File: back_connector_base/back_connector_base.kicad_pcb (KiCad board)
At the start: 2 copper layers, 102 x 77.7 mm, 10 parts, among them J1 Conn_01x12_Pin, J10 Conn_01x04_Socket, J2 Conn_01x16_Pin, J3 Conn_01x03_Socket, J4 Conn_01x03_Socket, J5 Conn_01x03_Socket, J6 Conn_01x03_Socket, J7 Conn_01x04_Socket, J8 Conn_01x04_Socket, J9 Conn_01x04_Socket

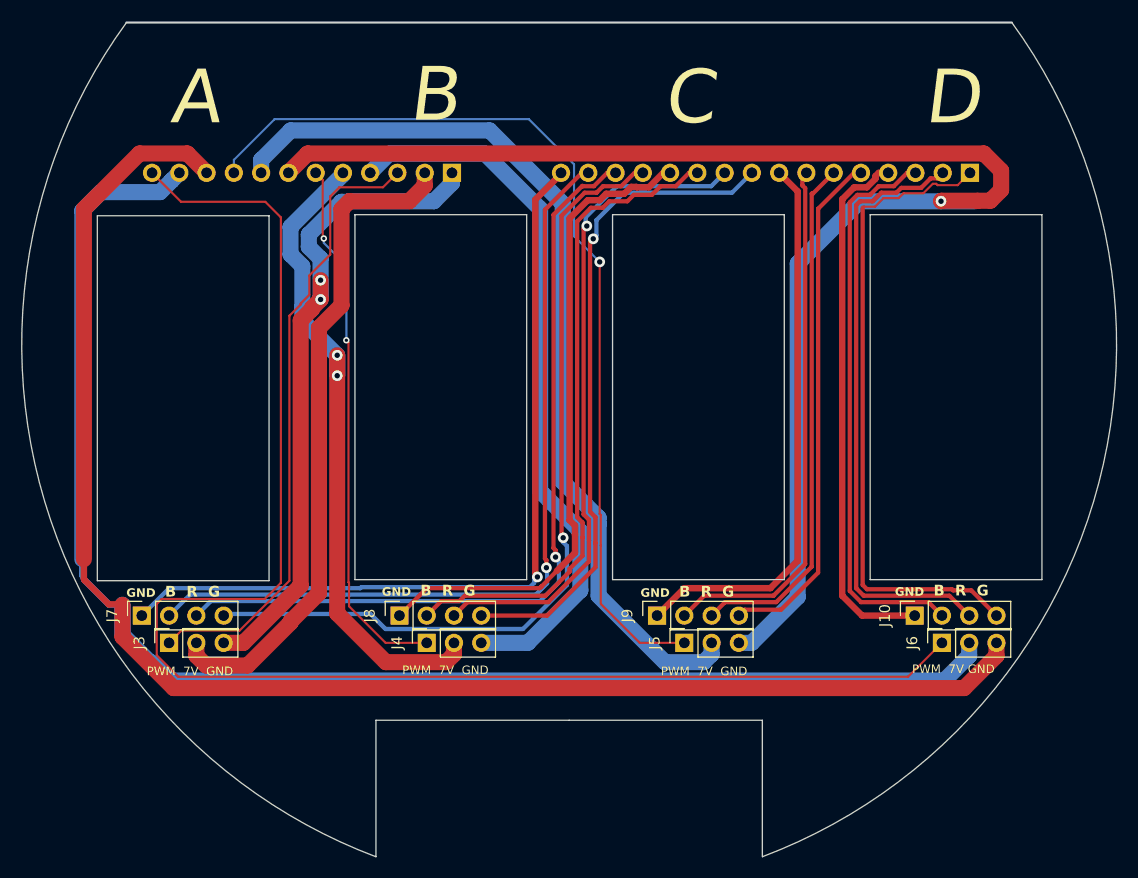
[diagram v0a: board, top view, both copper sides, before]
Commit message: ESC周りの配線用基板進捗
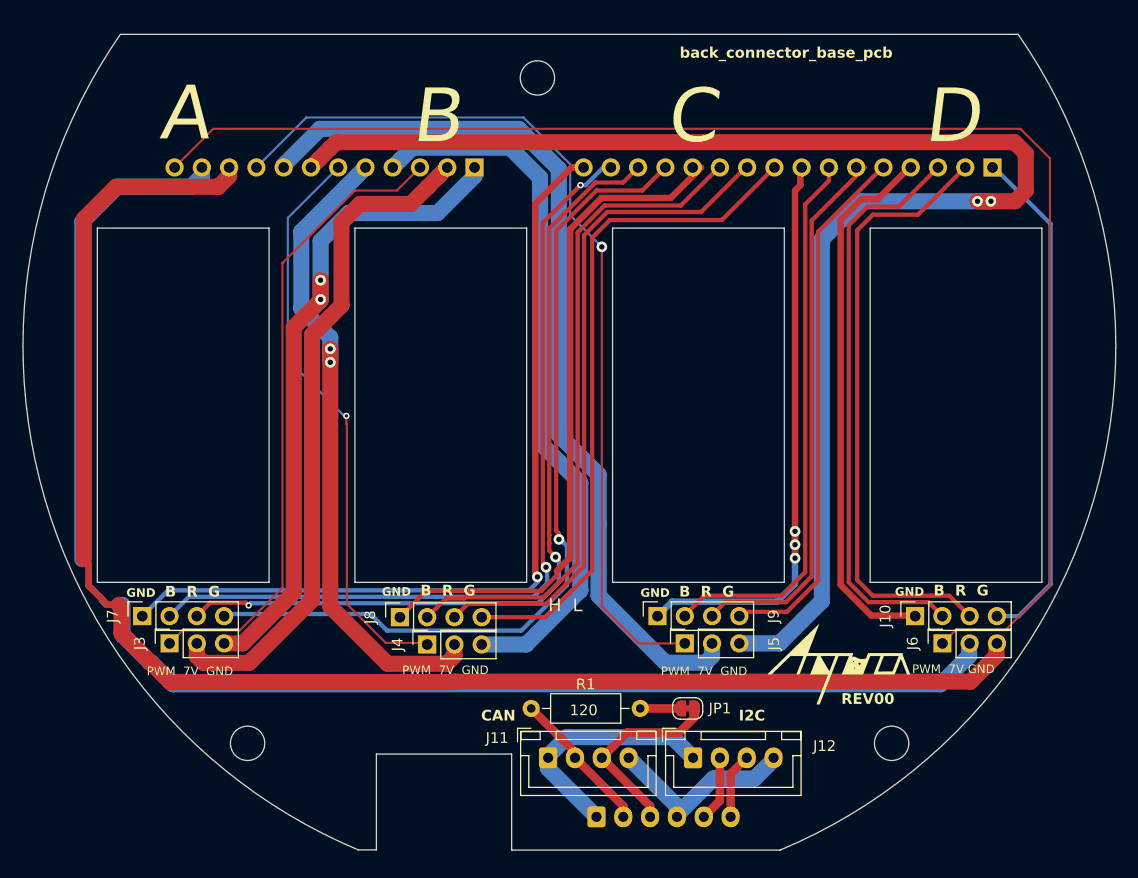
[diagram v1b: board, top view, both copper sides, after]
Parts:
- added G***: LOGO, specific_footprint_library:aqua_rogo, F.Cu at (96.4, 79.8)
- added H1: MountingHole, MountingHole:MountingHole_3.2mm_M3, F.Cu at (68.5, 25.3)
- added H2: MountingHole, MountingHole:MountingHole_3.2mm_M3, F.Cu at (41.5, 87.2)
- added H3: MountingHole, MountingHole:MountingHole_3.2mm_M3, F.Cu at (101.5, 87.2)
- added J11: Conn_01x04_Pin, Connector_JST:JST_XH_B4B-XH-A_1x04_P2.50mm_Vertical, F.Cu at (69.5, 88.6)
- added J12: Conn_01x04_Pin, Connector_JST:JST_XH_B4B-XH-A_1x04_P2.50mm_Vertical, F.Cu at (83.0, 88.6)
- added J13: Conn_01x06_Pin, Connector_JST:JST_XH_B6B-XH-A_1x06_P2.50mm_Vertical, B.Cu at (74.0, 94.1)
- added JP1: SolderJumper_2_Bridged, Jumper:SolderJumper-2_P1.3mm_Bridged_RoundedPad1.0x1.5mm, F.Cu at (82.5, 84.0)
- added R1: 120, Resistor_THT:R_Axial_DIN0207_L6.3mm_D2.5mm_P10.16mm_Horizontal, F.Cu at (78.1, 84.0)
- moved J2 2.16 mm to (110.9, 33.6)
- moved J1 2.16 mm to (62.6, 33.6)
- moved J4 0.16 mm to (58.2, 78.0)
- moved J8 0.16 mm to (55.7, 75.5)
- moved J7 0.07 mm to (31.7, 75.4)
- moved J10 0.07 mm to (103.7, 75.4)
- moved J9 0.07 mm to (79.7, 75.4)
- moved J5 0.07 mm to (82.2, 77.9)
- moved J6 0.07 mm to (106.2, 77.9)
- moved J3 0.07 mm to (34.2, 77.9)
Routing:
- net +5V: track 0.00 -> 22.6 mm
- net GND: track 0.00 -> 18.8 mm
- net Net-(J11-Pin_3): track 0.00 -> 18.4 mm
- net Net-(J11-Pin_2): track 0.00 -> 13.7 mm
- net D_G: track 60.2 -> 47.4 mm
- net Net-(J12-Pin_3): track 0.00 -> 6.12 mm
- net Net-(J12-Pin_2): track 0.00 -> 6.12 mm
- net Net-(J1-Pin_12): track 140.2 -> 136.2 mm
- net Net-(JP1-A): track 0.00 -> 3.77 mm
- net C_GND: track 52.1 -> 55.8 mm, vias 0 -> 3
- net Net-(J1-Pin_7): track 132.9 -> 136.6 mm, vias 1 -> 2
- net Net-(J1-Pin_9): track 87.9 -> 84.4 mm
- net Net-(J1-Pin_6): track 51.3 -> 54.0 mm, vias 2 -> 1
- net Net-(J1-Pin_11): track 135.1 -> 137.7 mm
- net A_G: track 78.2 -> 80.6 mm
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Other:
- board size 102 x 77.7 mm -> 101.8 x 76 mm
- board text added: "120"
- board text added: "7.19 3.25mm"
- board text added: "CAN"
- board text added: "H L"
- board text added: "I2C"
- board text added: "REV00"
- board text added: "back_connector_base_pcb"
